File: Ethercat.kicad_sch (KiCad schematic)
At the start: 49 parts, among them IC1 24AA32AF, J1 RJ45_Amphenol_RJMG1BD3B8K1ANR, J2 RJ45_Amphenol_RJMG1BD3B8K1ANR, Y1 25Mhz

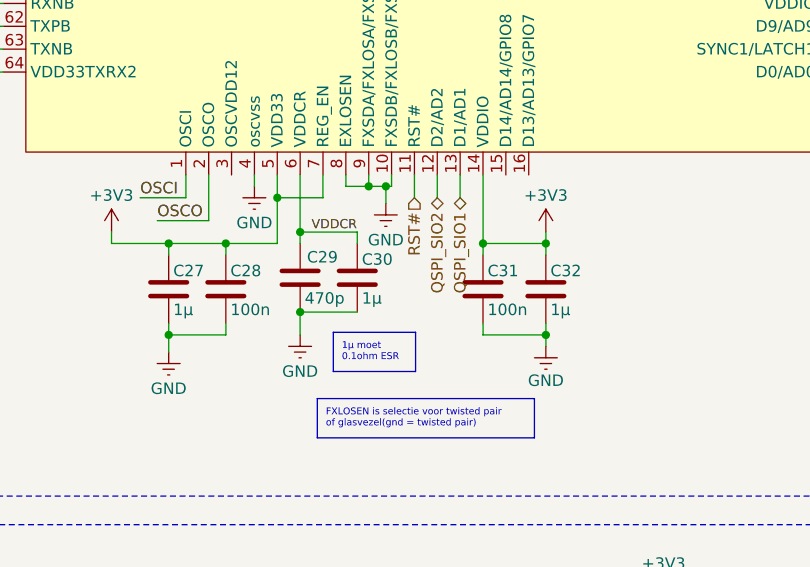
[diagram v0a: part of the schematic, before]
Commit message: schema's finalized
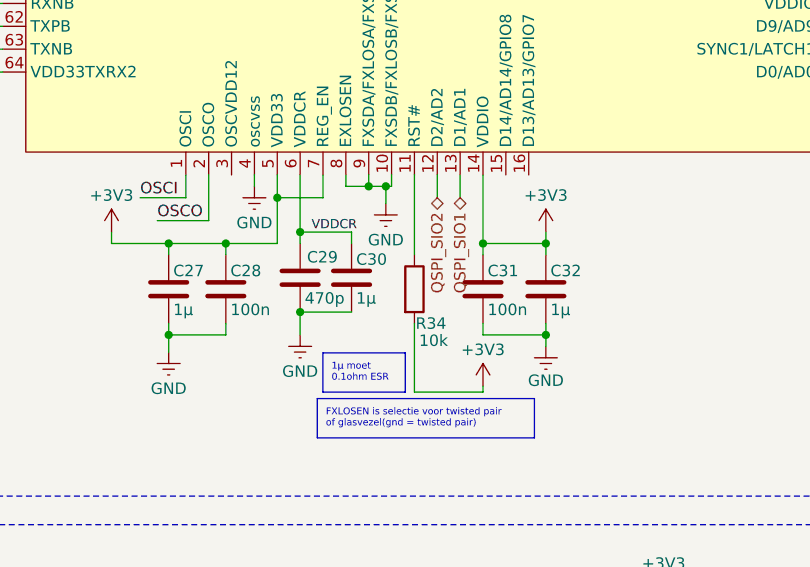
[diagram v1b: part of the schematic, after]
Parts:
- added R34: 10k, Resistor_SMD:R_0603_1608Metric, symbol Device:R
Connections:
- net +3V3: now also R34.2
- net RST#: no longer names the net of U2.11 (RST#)
- net RST#: now also R34.1
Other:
- moved on the sheet: C30
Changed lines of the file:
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@@
 	(text_box "1µ moet 0.1ohm ESR\n"
 		(exclude_from_sim no)
-		(at 139.573 190.206 0)
+		(at 138.43 192.492 0)
 		(size 9.144 4.358)
 		(margins 0.9525 0.9525 0.9525 0.9525)
@@
 	(wire
 		(pts
+			(xy 148.59 172.72) (xy 148.59 181.61)
+		)
+		(stroke
+			(width 0)
+			(type default)
+		)
+	)
+	(wire
+		(pts
 			(xy 52.07 151.13) (xy 52.07 152.4)
 		)
@@
 	(wire
 		(pts
-			(xy 142.24 180.34) (xy 142.24 179.07)
+			(xy 141.605 180.34) (xy 141.605 179.07)
+		)
+		(stroke
+			(width 0)
+			(type default)
+		)
+	)
+	(wire
+		(pts
+			(xy 156.21 196.85) (xy 156.21 196.215)
 		)
 		(stroke
@@
 	(wire
 		(pts
+			(xy 148.59 196.85) (xy 156.21 196.85)
+		)
+		(stroke
+			(width 0)
+			(type default)
+		)
+	)
+	(wire
+		(pts
 			(xy 89.535 163.83) (xy 89.535 162.56)
 		)
@@
 	(wire
 		(pts
-			(xy 135.89 187.96) (xy 142.24 187.96)
+			(xy 135.89 187.96) (xy 141.605 187.96)
 		)
 		(stroke
@@
 	(wire
 		(pts
+			(xy 148.59 189.23) (xy 148.59 196.85)
+		)
+		(stroke
+			(width 0)
+			(type default)
+		)
+	)
+	(wire
+		(pts
 			(xy 303.53 151.765) (xy 303.53 142.875)
 		)
@@
 	(wire
 		(pts
-			(xy 135.89 179.07) (xy 142.24 179.07)
+			(xy 135.89 179.07) (xy 141.605 179.07)
 		)
 		(stroke
@@
 	(wire
 		(pts
-			(xy 148.59 172.72) (xy 148.59 175.26)
-		)
-		(stroke
-			(width 0)
-			(type default)
-		)
-	)
-	(wire
-		(pts
 			(xy 121.285 192.405) (xy 121.285 190.5)
 		)
@@
 		)
 	)
-	(hierarchical_label "RST#"
-		(shape input)
-		(at 148.59 175.26 270)
-		(effects
-			(font
-				(size 1.27 1.27)
-			)
-			(justify right)
-		)
-	)
 	(hierarchical_label "IRQ"
 		(shape output)
@@
 	)
 	(symbol
+		(lib_id "power:+3V3")
+		(at 156.21 196.215 0)
+		(unit 1)
+		(body_style 1)
+		(exclude_from_sim no)
+		(in_bom yes)
+		(on_board yes)
+		(in_pos_files yes)
+		(dnp no)
+		(property "Reference" "#PWR0119"
+			(at 156.21 200.025 0)
+			(hide yes)
+			(show_name no)
+			(do_not_autoplace no)
+			(effects
+				(font
+					(size 1.27 1.27)
+				)
+			)
+		)
+		(property "Value" "+3V3"
+			(at 156.21 192.151 0)
+			(show_name no)
+			(do_not_autoplace no)
+			(effects
+				(font
+					(size 1.27 1.27)
+				)
+			)
+		)
+		(property "Footprint" "Package_DIP:DIP-24_W7.62mm"
+			(at 156.21 196.215 0)
+			(hide yes)
+			(show_name no)
+			(do_not_autoplace no)
+			(effects
+				(font
+					(size 1.27 1.27)
+				)
+			)
+		)
+		(property "Datasheet" ""
+			(at 156.21 196.215 0)
+			(hide yes)
+			(show_name no)
+			(do_not_autoplace no)
+			(effects
+				(font
+					(size 1.27 1.27)
+				)
+			)
+		)
+		(property "Description" "Power symbol creates a global label with name \"+3V3\""
+			(at 156.21 196.215 0)
+			(hide yes)
+			(show_name no)
+			(do_not_autoplace no)
+			(effects
+				(font
+					(size 1.27 1.27)
+				)
+			)
+		)
+		(pin "1"
+		)
+		(instances
+			(project "ESC_PLC"
+				(path "/5bd3bb6f-fe53-443c-806c-077e2bbb5d14/f038ea58-2b1a-4d87-b3c8-8d32ce4ec05b"
+					(reference "#PWR0119")
+					(unit 1)
+				)
+			)
+		)
+	)
+	(symbol
 		(lib_id "EEPROM:579-24LC32AFT-I/SN")
 		(at 273.05 144.145 0)
@@
 	)
 	(symbol
+		(lib_id "Device:R")
+		(at 148.59 185.42 0)
+		(unit 1)
+		(body_style 1)
+		(exclude_from_sim no)
+		(in_bom yes)
+		(on_board yes)
+		(in_pos_files yes)
+		(dnp no)
+		(property "Reference" "R34"
+			(at 148.717 189.23 0)
+			(show_name no)
+			(do_not_autoplace no)
+			(effects
+				(font
+					(size 1.27 1.27)
+				)
+				(justify left)
+			)
+		)
+		(property "Value" "10k"
+			(at 149.098 191.135 0)
+			(show_name no)
+			(do_not_autoplace no)
+			(effects
+				(font
+					(size 1.27 1.27)
+				)
+				(justify left)
+			)
+		)
+		(property "Footprint" "Resistor_SMD:R_0603_1608Metric"
+			(at 146.812 185.42 90)
+			(hide yes)
+			(show_name no)
+			(do_not_autoplace no)
+			(effects
+				(font
+					(size 1.27 1.27)
+				)
+			)
+		)
+		(property "Datasheet" ""
+			(at 148.59 185.42 0)
+			(hide yes)
+			(show_name no)
+			(do_not_autoplace no)
+			(effects
+				(font
+					(size 1.27 1.27)
+				)
+			)
+		)
+		(property "Description" "Resistor"
+			(at 148.59 185.42 0)
+			(hide yes)
+			(show_name no)
+			(do_not_autoplace no)
+			(effects
+				(font
+					(size 1.27 1.27)
+				)
+			)
+		)
+		(pin "2"
+		)
+		(pin "1"
+		)
+		(instances
+			(project "ESC_PLC"
+				(path "/5bd3bb6f-fe53-443c-806c-077e2bbb5d14/f038ea58-2b1a-4d87-b3c8-8d32ce4ec05b"
+					(reference "R34")
+					(unit 1)
+				)
+			)
+		)
+	)
+	(symbol
 		(lib_id "power:+3V3")
 		(at 114.935 179.07 0)
@@
 	(symbol
 		(lib_id "Device:C")
-		(at 142.24 184.15 0)
+		(at 141.605 184.15 0)
 		(unit 1)
 		(body_style 1)
@@
 		(dnp no)
 		(property "Reference" "C30"
-			(at 142.748 182.118 0)
+			(at 142.113 182.118 0)
 			(show_name no)
 			(do_not_autoplace no)
@@
 		)
 		(property "Value" "1µ"
-			(at 142.748 186.436 0)
+			(at 142.113 186.436 0)
 			(show_name no)
 			(do_not_autoplace no)
@@
 		)
 		(property "Footprint" "Capacitor_SMD:C_0603_1608Metric"
-			(at 143.2052 187.96 0)
+			(at 142.5702 187.96 0)
 			(hide yes)
 			(show_name no)
@@
 		)
 		(property "Datasheet" ""
-			(at 142.24 184.15 0)
+			(at 141.605 184.15 0)
 			(hide yes)
 			(show_name no)
@@
 		)
 		(property "Description" "Unpolarized capacitor"
-			(at 142.24 184.15 0)
+			(at 141.605 184.15 0)
 			(hide yes)
 			(show_name no)
